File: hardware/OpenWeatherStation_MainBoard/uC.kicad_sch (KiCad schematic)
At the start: 2 parts, among them U1 STM32F107VCTx

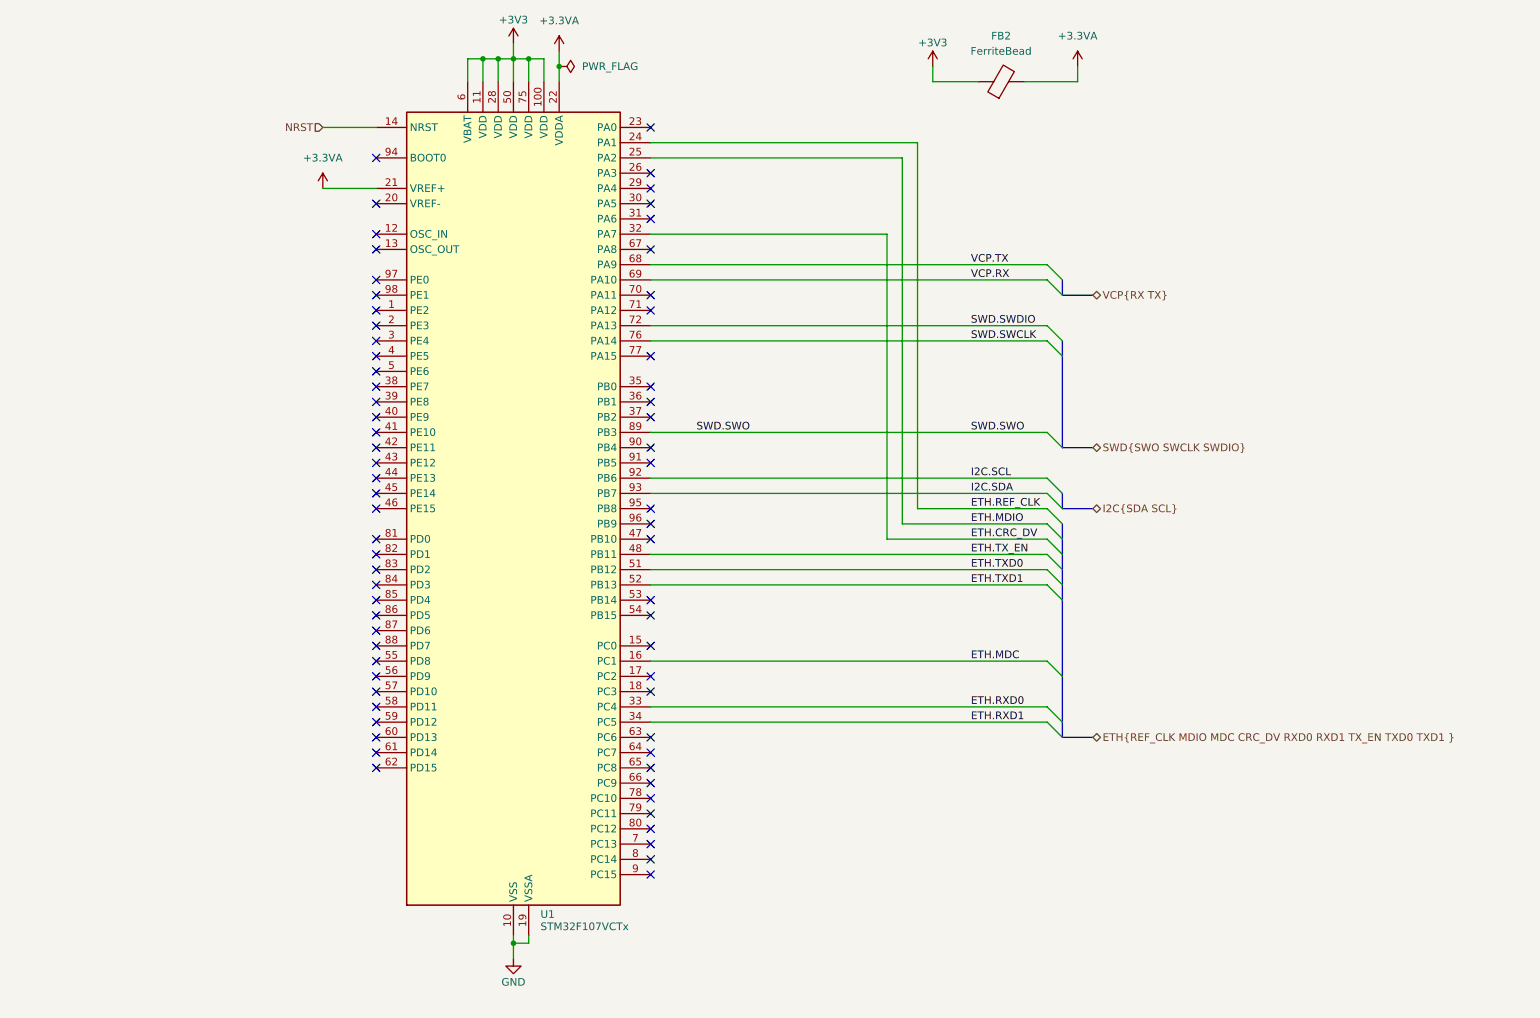
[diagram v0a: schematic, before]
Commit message: udpate pcb design
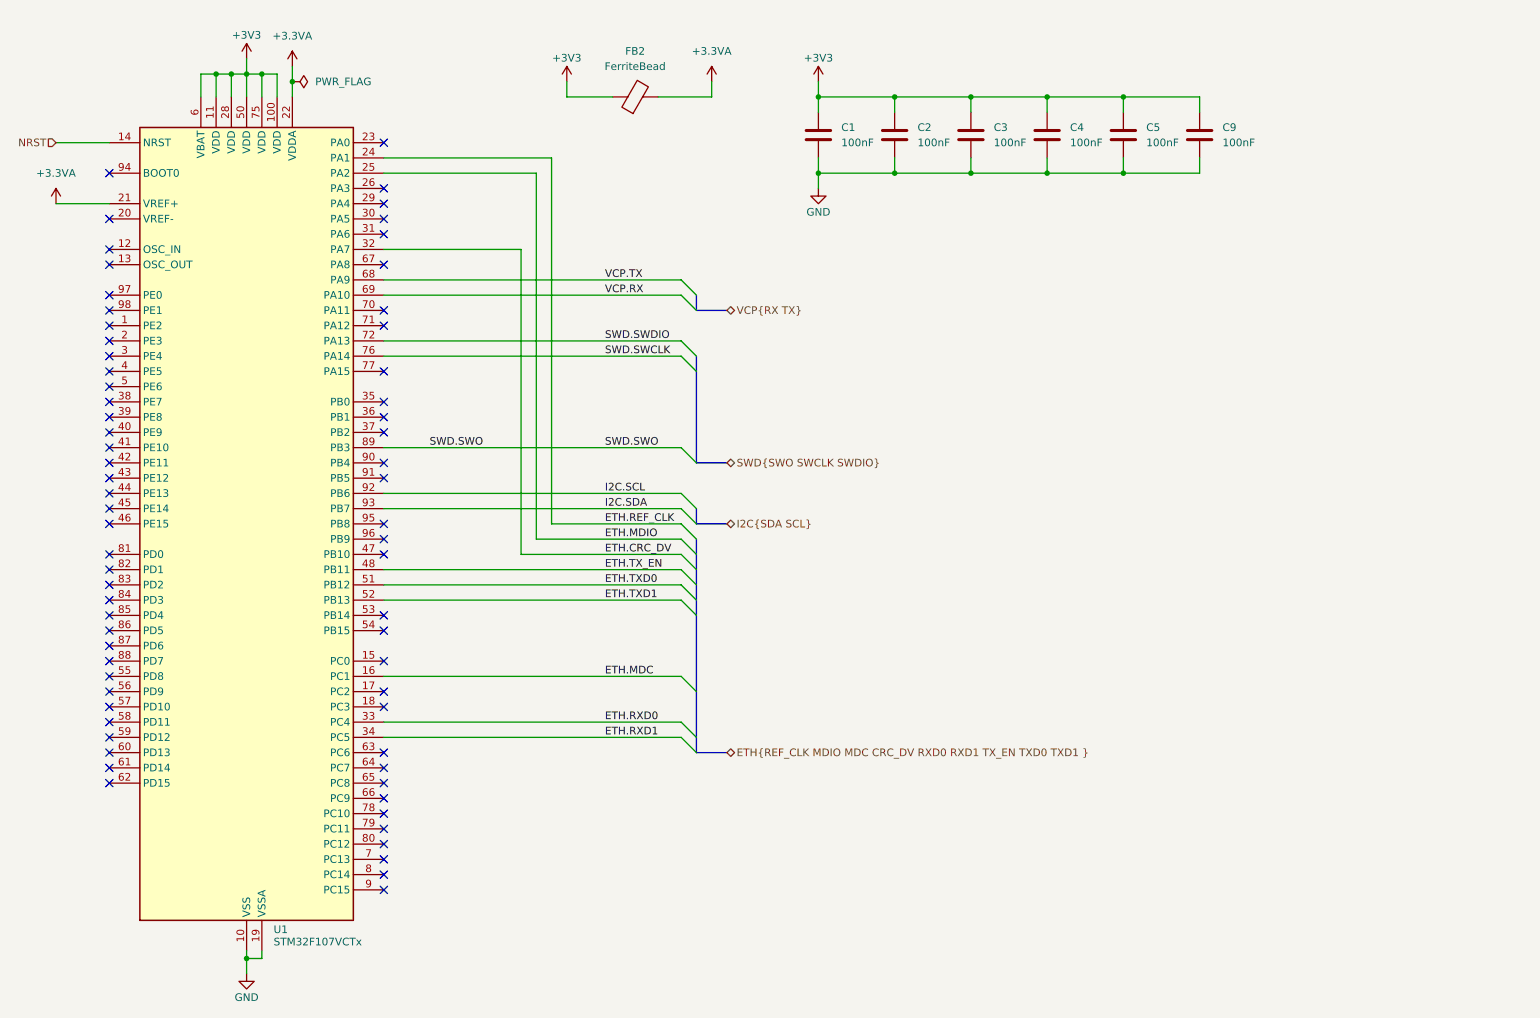
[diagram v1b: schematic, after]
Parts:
- added C1, C2, C3, C4, C5, C9: 100nF, Capacitor_SMD:C_0603_1608Metric, symbol Device:C
- FB2: footprint (none) -> Capacitor_SMD:C_0603_1608Metric
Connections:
- net +3V3: now also C1.1, C2.1, C3.1, C4.1, C5.1, C9.1
- net GND: now also C1.2, C2.2, C3.2, C4.2, C5.2, C9.2
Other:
- moved on the sheet: FB2, U1
